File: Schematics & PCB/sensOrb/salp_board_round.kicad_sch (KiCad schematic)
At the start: 78 parts, among them J1 ATTINY3226, J10 POWER, J2 READ/WRITE, J3 READ/WRITE, J4 Conn_01x03, J8 ATTINY3226, J9 POWER_JUMPER, Q1 IRLML6402, Q2 IRLML6402, U1 LD1117S33TR, U2 PN5321A3HN/C106_55, U3 ATtiny3226-S, U4 TP4057, U6 DW01A, Y2 27.12 MHz

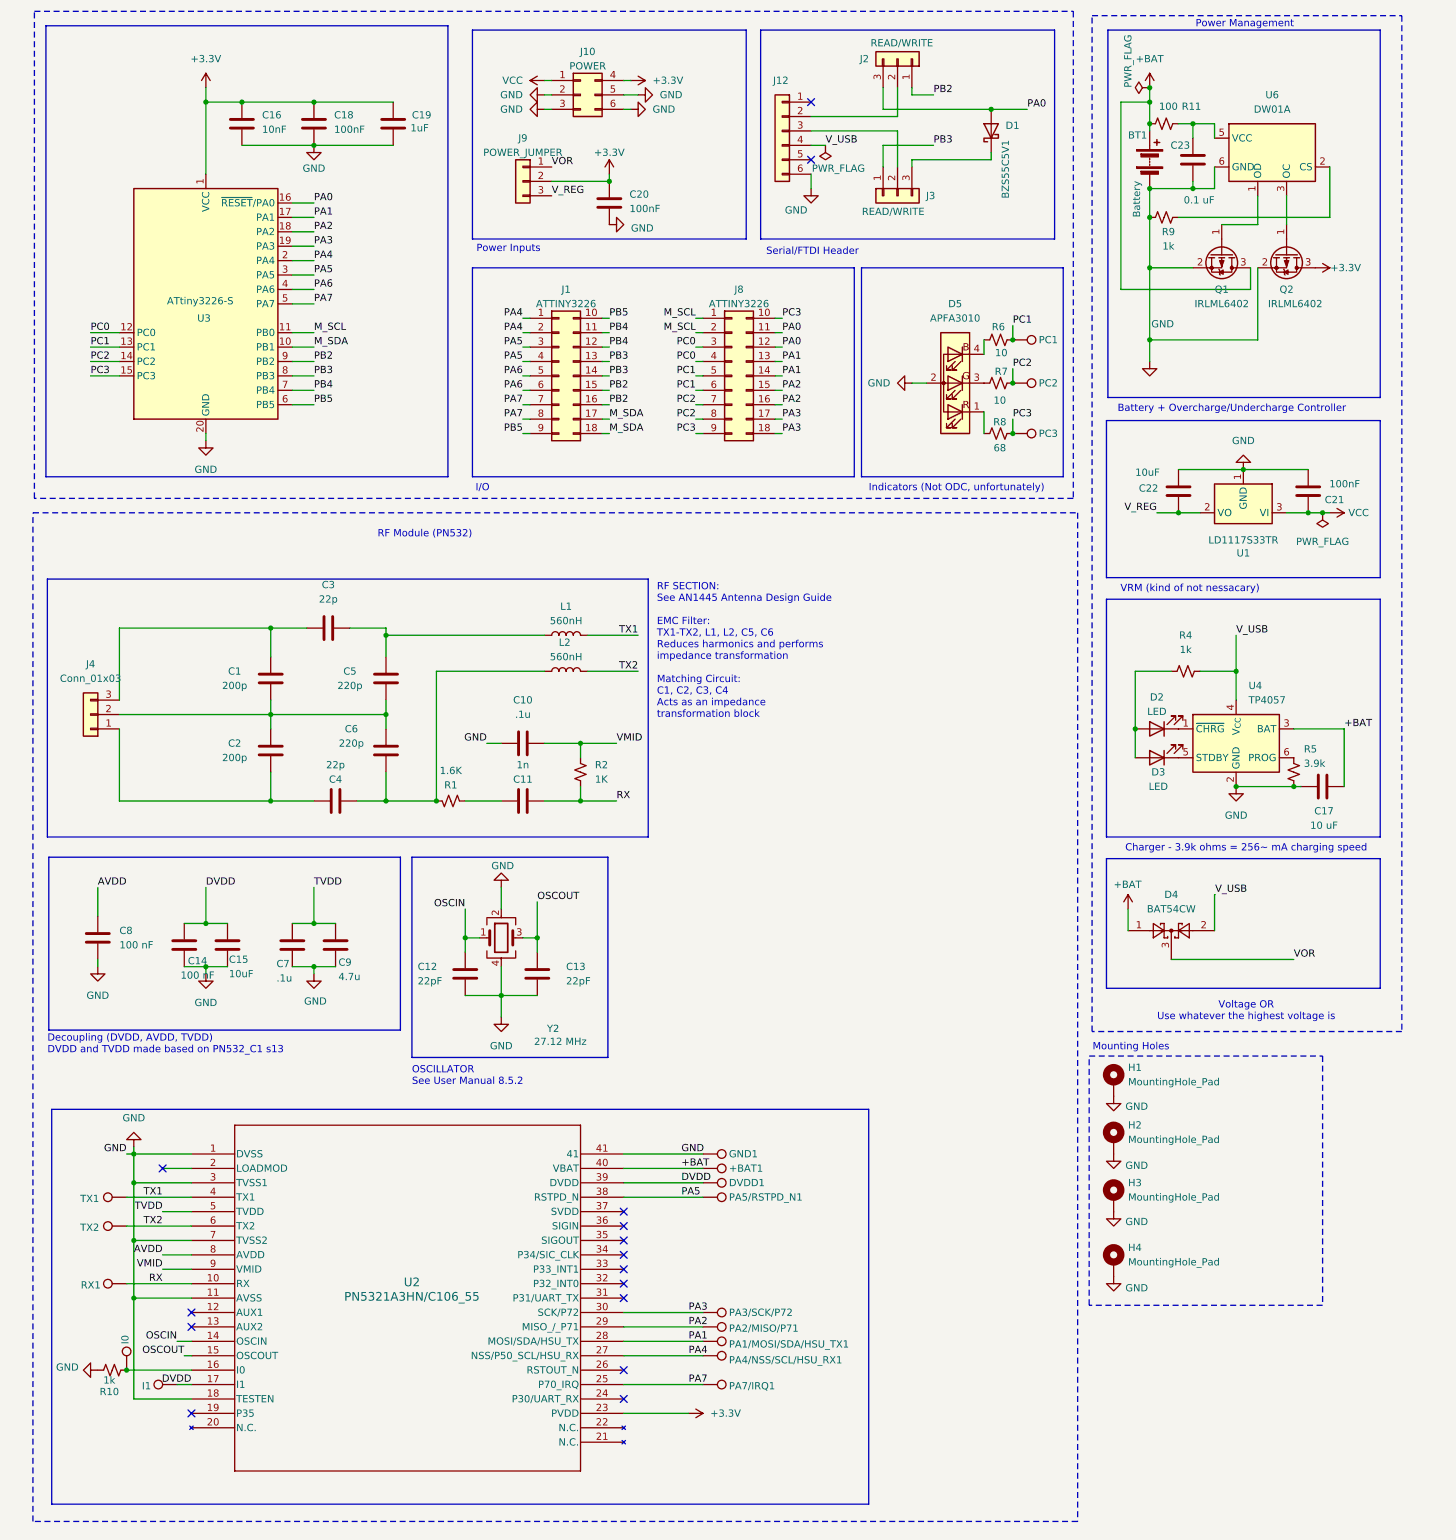
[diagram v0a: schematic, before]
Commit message: Updated SCH
Schematic update: new power regulator layout, communication protocol jumper selectors
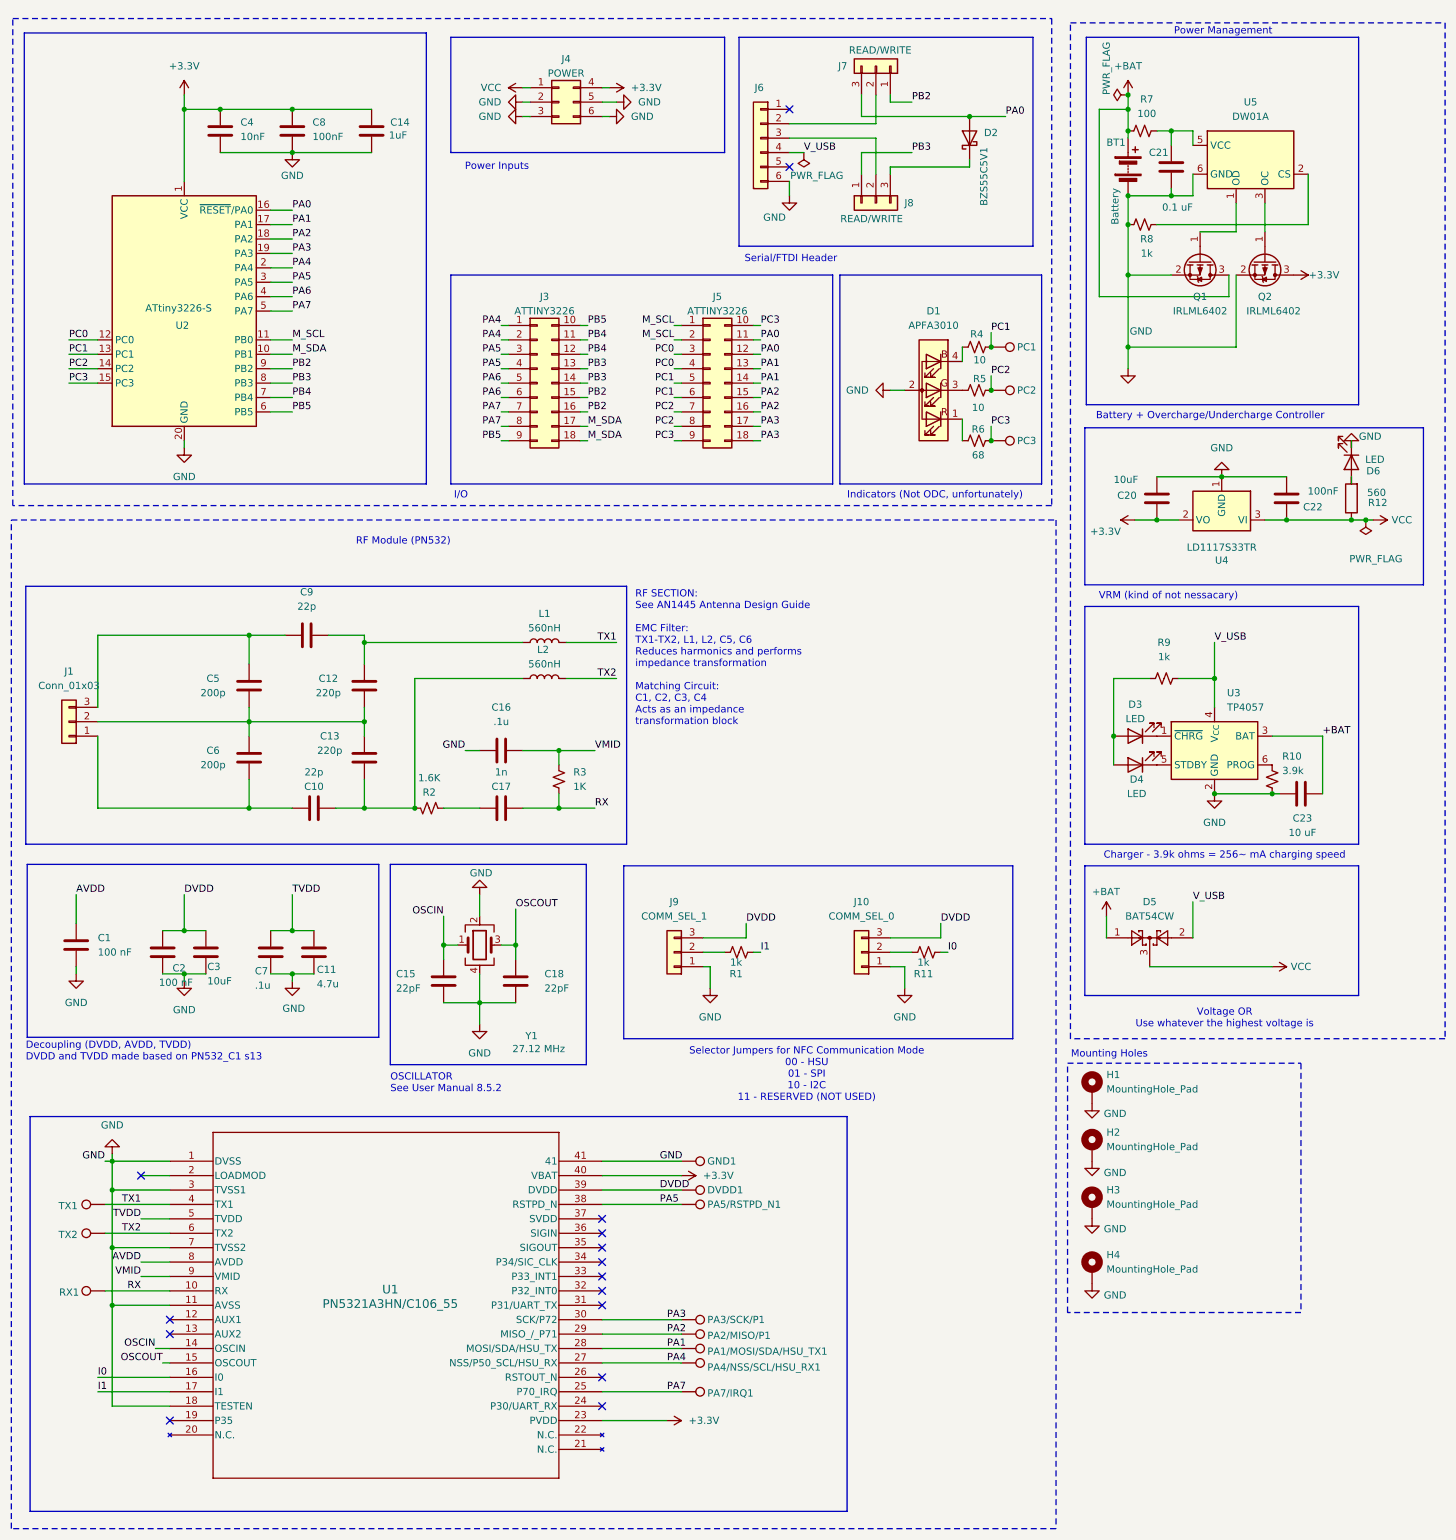
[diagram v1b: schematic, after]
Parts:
- removed +BAT1, I0, I1, PA2/MISO/P71, PA3/SCK/P72: TestPoint, TestPoint:TestPoint_Pad_D1.0mm, symbol Connector:TestPoint
- removed C19: 1uF, Capacitor_SMD:C_0805_2012Metric_Pad1.18x1.45mm_HandSolder, symbol Device:C
- removed D1: BZS55C5V1, Diode_SMD:D_1206_3216Metric_Pad1.42x1.75mm_HandSolder, symbol Device:D_Schottky
- removed D2: LED, LED_SMD:LED_0805_2012Metric, symbol Device:LED
- removed D4: BAT54CW, Package_TO_SOT_SMD:SOT-323_SC-70, symbol Diode:BAT54CW
- removed D5: APFA3010, LED_SMD:LED_Kingbright_APFA3010_3x1.5mm_Horizontal, symbol LED:APFA3010
- removed J1, J8: ATTINY3226, Connector_PinSocket_2.54mm:PinSocket_2x09_P2.54mm_Vertical, symbol Connector_Generic:Conn_02x09_Top_Bottom
- removed J10: POWER, Connector_PinSocket_2.54mm:PinSocket_2x03_P2.54mm_Vertical, symbol Connector_Generic:Conn_02x03_Top_Bottom
- removed J12: ~, Connector_PinHeader_2.54mm:PinHeader_1x06_P2.54mm_Horizontal, symbol Connector_Generic:Conn_01x06
- removed J2, J3: READ/WRITE, Connector_PinHeader_2.54mm:PinHeader_1x03_P2.54mm_Vertical, symbol Connector_Generic:Conn_01x03
- removed J4: Conn_01x03, Connector_PinHeader_2.54mm:PinHeader_1x03_P2.54mm_Horizontal, symbol Connector_Generic:Conn_01x03
- removed U1: LD1117S33TR, Package_TO_SOT_SMD:SOT-223-3_TabPin2, symbol Regulator_Linear:LD1117S33TR_SOT223
- removed U2: PN5321A3HN/C106_55, PN532:QFN40G-0.5-6X6MM, symbol Orb_library:PN5321A3HN_C106_55
- removed U3: ATtiny3226-S, Package_SO:SOIC-20W_7.5x12.8mm_P1.27mm, symbol MCU_Microchip_ATtiny:ATtiny3226-S
- removed U4: TP4057, Package_TO_SOT_SMD:TSOT-23-6, symbol Battery_Management:TP4057
- removed U6: DW01A, Package_TO_SOT_SMD:SOT-23-6, symbol Battery_Management:DW01A
- removed Y2: 27.12 MHz, Crystal:Crystal_SMD_SeikoEpson_TSX3225-4Pin_3.2x2.5mm_HandSoldering, symbol Device:Crystal_GND24
- added D1: APFA3010, LED_SMD:LED_Kingbright_APFA3010_3x1.5mm_Horizontal, symbol LED:APFA3010
- added D2: BZS55C5V1, Diode_SMD:D_1206_3216Metric_Pad1.42x1.75mm_HandSolder, symbol Device:D_Schottky
- added D4: LED, LED_SMD:LED_0805_2012Metric, symbol Device:LED
- added D5: BAT54CW, Package_TO_SOT_SMD:SOT-323_SC-70, symbol Diode:BAT54CW
- added D6: LED, LED_SMD:LED_0603_1608Metric_Pad1.05x0.95mm_HandSolder, symbol Device:LED
- added J1: Conn_01x03, Connector_PinHeader_2.54mm:PinHeader_1x03_P2.54mm_Horizontal, symbol Connector_Generic:Conn_01x03
- added J10: COMM_SEL_0, Connector_PinHeader_2.54mm:PinHeader_1x03_P2.54mm_Horizontal, symbol Connector_Generic:Conn_01x03
- added J3, J5: ATTINY3226, Connector_PinSocket_2.54mm:PinSocket_2x09_P2.54mm_Vertical, symbol Connector_Generic:Conn_02x09_Top_Bottom
- added J4: POWER, Connector_PinSocket_2.54mm:PinSocket_2x03_P2.54mm_Vertical, symbol Connector_Generic:Conn_02x03_Top_Bottom
- added J6: ~, Connector_PinHeader_2.54mm:PinHeader_1x06_P2.54mm_Horizontal, symbol Connector_Generic:Conn_01x06
- added J7, J8: READ/WRITE, Connector_PinHeader_2.54mm:PinHeader_1x03_P2.54mm_Vertical, symbol Connector_Generic:Conn_01x03
- added PA2/MISO/P1, PA3/SCK/P1: TestPoint, TestPoint:TestPoint_Pad_D1.0mm, symbol Connector:TestPoint
- added R12: 560, Resistor_SMD:R_0805_2012Metric_Pad1.20x1.40mm_HandSolder, symbol Device:R
- added R3: 1K, Resistor_SMD:R_0805_2012Metric_Pad1.20x1.40mm_HandSolder, symbol Device:R_Small_US
- added U1: PN5321A3HN/C106_55, PN532:QFN40G-0.5-6X6MM, symbol Orb_library:PN5321A3HN_C106_55
- added U2: ATtiny3226-S, Package_SO:SOIC-20W_7.5x12.8mm_P1.27mm, symbol MCU_Microchip_ATtiny:ATtiny3226-S
- added U3: TP4057, Package_TO_SOT_SMD:TSOT-23-6, symbol Battery_Management:TP4057
- added U4: LD1117S33TR, Package_TO_SOT_SMD:SOT-223-3_TabPin2, symbol Regulator_Linear:LD1117S33TR_SOT223
- added U5: DW01A, Package_TO_SOT_SMD:SOT-23-6, symbol Battery_Management:DW01A
- added Y1: 27.12 MHz, Crystal:Crystal_SMD_SeikoEpson_TSX3225-4Pin_3.2x2.5mm_HandSoldering, symbol Device:Crystal_GND24
- C1, C2: value 200p -> 100 nF
- C10: value .1u -> 22p
- C11: value 1n -> 4.7u
- C12, C13: value 22pF -> 220p
- C14: value 100 nF -> 1uF
- C15: value 10uF -> 22pF
- C16: value 10nF -> .1u
- C17: value 10 uF -> 1n
- C18: value 100nF -> 22pF
- C20: value 100nF -> 10uF
- C21: value 100nF -> 0.1 uF
- C22: value 10uF -> 100nF
- C23: value 0.1 uF -> 10 uF
- C3: value 22p -> 10uF
- C4: value 22p -> 10nF
- C5, C6: value 220p -> 200p
- C8: value 100 nF -> 100nF
- C9: value 4.7u -> 22p
- J9: value POWER_JUMPER -> COMM_SEL_1; footprint Connector_PinHeader_2.54mm:PinHeader_1x03_P2.54mm_Vertical -> Connector_PinHeader_2.54mm:PinHeader_1x03_P2.54mm_Horizontal
- R1: value 1.6K -> 1k
- R10: value 1k -> 3.9k
- R11: value 100 -> 1k
- R2: value 1K -> 1.6K
- R4: value 1k -> 10
- R5: value 3.9k -> 10
- R6: value 10 -> 68
- R7: value 10 -> 100
- R8: value 68 -> 1k
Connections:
- net VOR is gone; now on net GND: J9.1 (Pin_1)
- net +3.3V: now also C14.1, C4.1, C8.1, J4.4 (Pin_4), U1.23 (PVDD), U1.40 (VBAT), U2.1 (VCC), U4.2 (VO); no longer C16.1, C18.1, J9.2 (Pin_2)
- net +BAT: now also C23.2, R7.1, D5.1, U3.3 (BAT); no longer C17.2, R11.1
- net AVDD: now also C1.1, U1.8 (AVDD); no longer C8.1
- net DVDD: now also C2.1, C3.1, J9.3 (Pin_3), J10.3 (Pin_3), U1.39 (DVDD); no longer C14.1, C15.1
- net GND: now also C1.2, C11.2, C2.2, C21.1, C3.2, C4.2, R8.1, D1.2 (A), D6.1 (K), J10.1 (Pin_1), J4.2 (Pin_2), J4.3 (Pin_3), J4.5 (Pin_5), J4.6 (Pin_6), J6.6 (Pin_6), U1.1 (DVSS), U1.11 (AVSS), U1.18 (TESTEN), U1.3 (TVSS1), U1.41, U1.7 (TVSS2), U2.20 (GND), U3.2 (GND), U4.1 (GND), U5.6 (GND), Y1.2, Y1.4; no longer C10.2, C12.2, C13.2, C17.1, C21.2, C9.2, R5.1, R9.1
- net M_SCL: now also J5.1 (Pin_1), J5.2 (Pin_2), U2.11 (PB0)
- net M_SDA: now also J3.17 (Pin_17), J3.18 (Pin_18), U2.10 (PB1)
- net OSCIN: now also C15.1, U1.14 (OSCIN), Y1.1; no longer C12.1
- net OSCOUT: now also C18.1, U1.15 (OSCOUT), Y1.3; no longer C13.1
- net PA0: now also D2.2 (A), J5.11 (Pin_11), J5.12 (Pin_12), J7.3 (Pin_3), U2.16 (~{RESET}/PA0)
- net PA1: now also J5.13 (Pin_13), J5.14 (Pin_14), U1.28 (MOSI/SDA/HSU_TX), U2.17 (PA1)
- net PA2: now also J5.15 (Pin_15), J5.16 (Pin_16), PA2/MISO/P1.1, U1.29 (MISO_/_P71), U2.18 (PA2)
- net PA3: now also J5.17 (Pin_17), J5.18 (Pin_18), PA3/SCK/P1.1, U1.30 (SCK/P72), U2.19 (PA3)
- net PA4: now also J3.1 (Pin_1), J3.2 (Pin_2), U1.27 (NSS/P50_SCL/HSU_RX), U2.2 (PA4)
- net PA5: now also J3.3 (Pin_3), J3.4 (Pin_4), U1.38 (RSTPD_N), U2.3 (PA5)
- net PA6: now also J3.5 (Pin_5), J3.6 (Pin_6), U2.4 (PA6)
- net PA7: now also J3.7 (Pin_7), J3.8 (Pin_8), U1.25 (P70_IRQ), U2.5 (PA7)
- net PB2: now also J3.15 (Pin_15), J3.16 (Pin_16), J7.1 (Pin_1), U2.9 (PB2)
- net PB3: now also J3.13 (Pin_13), J3.14 (Pin_14), J8.1 (Pin_1), U2.8 (PB3)
- net PB4: now also J3.11 (Pin_11), J3.12 (Pin_12), U2.7 (PB4)
- net PB5: now also J3.10 (Pin_10), J3.9 (Pin_9), U2.6 (PB5)
- net PC0: now also J5.3 (Pin_3), J5.4 (Pin_4), U2.12 (PC0)
- net PC1: now also R4.2, J5.5 (Pin_5), J5.6 (Pin_6), U2.13 (PC1); no longer R6.2
- net PC2: now also R5.2, J5.7 (Pin_7), J5.8 (Pin_8), U2.14 (PC2); no longer R7.2
- net PC3: now also R6.2, J5.10 (Pin_10), J5.9 (Pin_9), U2.15 (PC3); no longer R8.2
- net RX: now also C17.2, R3.2, U1.10 (RX); no longer C11.2, R2.2
- net TVDD: now also C11.1, U1.5 (TVDD); no longer C9.1
- net TX1: now also U1.4 (TX1)
- net TX2: now also U1.6 (TX2)
- net VCC: now also C22.1, D5.3, J4.1 (Pin_1), R12.1, U4.3 (VI); no longer C21.1
- net VMID: now also C16.1, R3.1, U1.9 (VMID); no longer C10.1, R2.1
- net V_USB: now also R9.2, D5.2, J6.4 (Pin_4), U3.4 (V_{CC}); no longer R4.2
- net at C5.2, C6.1: now also C12.2, C13.1, J1.2 (Pin_2); no longer C1.2, C2.1
- net I1: now reaches R1.2
- net I1: now also U1.17 (I1); no longer C11.1
- net I0: now reaches R11.2
- net I0: now also U1.16 (I0); no longer C23.2
- net at R10.2: now also U3.6 (PROG)
- net at D3.2 (A): now also R9.1, D4.2 (A); no longer R4.1
- net at R6.1: now also D1.1 (R)
- net at Q1.1 (G): now also U5.1 (OD)
- net at Q2.1 (G): now also U5.3 (OC)
- net at D3.1 (K): now also U3.1 (~{CHRG})
- removed net V_REG: C22.1, J9.3 (Pin_3)
- new net: D4.1 (K), U3.5 (STDBY)
- new net: C10.1, C6.2, J1.1 (Pin_1)
- new net: C10.2, C13.2, L2.1, R2.1
- new net: C12.1, C9.2, L1.1
- new net: J9.2 (Pin_2), R1.1
- new net: C17.1, R2.2
- new net: D1.3 (G), R5.1
- new net: D1.4 (B), R4.1
- new net: C5.1, C9.1, J1.3 (Pin_3)
- new net: C21.2, R7.2, U5.5 (VCC)
- new net: J6.2 (Pin_2), J7.2 (Pin_2)
- new net: J10.2 (Pin_2), R11.1
- new net: D2.1 (K), J8.3 (Pin_3)
- new net: J6.3 (Pin_3), J8.2 (Pin_2)
- new net: R8.2, U5.2 (CS)
- new net: D6.2 (A), R12.2
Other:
- note added: "Selector Jumpers for NFC Communication Mode 00 - HSU 01 - SPI 10 - I2C 11 - RESERVED (NOT USED)"
- company: (none) -> Jack Cunningham
- title: (none) -> SALP_NFC_Round
